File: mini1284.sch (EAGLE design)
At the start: 25 parts, among them U1 ATmega1284P-AU

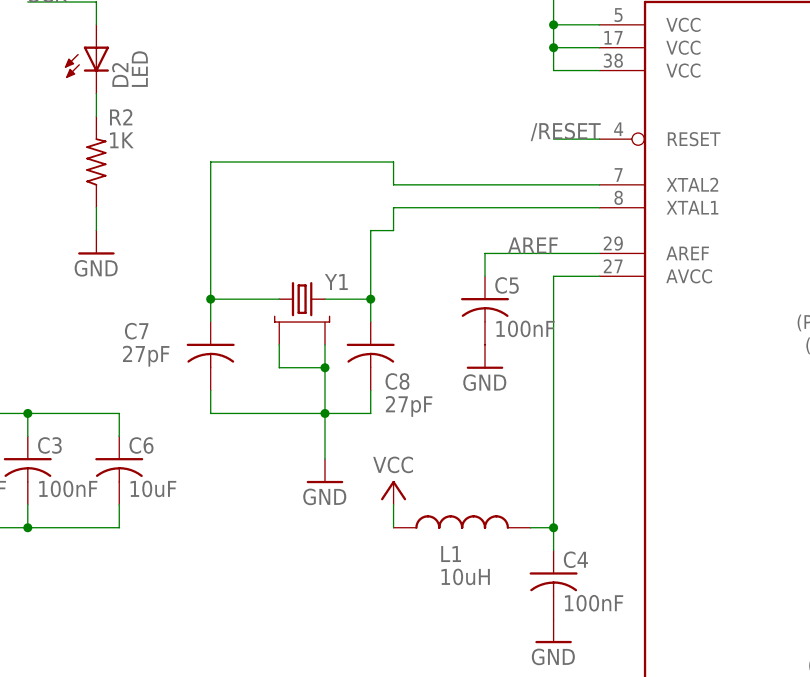
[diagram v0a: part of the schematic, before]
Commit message: Minor tweaks.
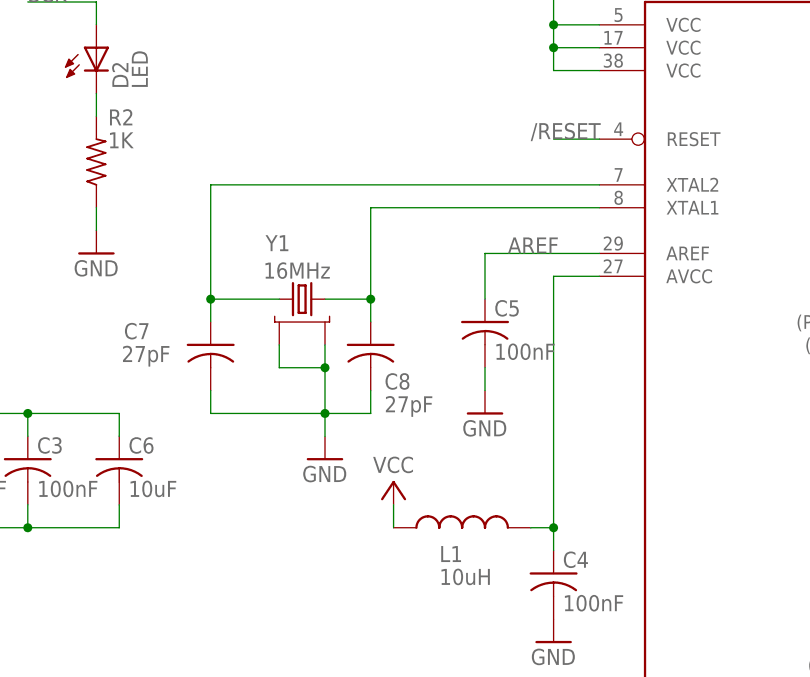
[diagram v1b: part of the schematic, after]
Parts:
- Y1: value (none) -> 16MHz
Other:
- moved on the sheet: C5
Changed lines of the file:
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@@
 <part name="D2" library="_jc" deviceset="LED" device="D0805A" value="LED"/>
 <part name="GND7" library="SparkFun" deviceset="GND" device=""/>
-<part name="Y1" library="_jc" deviceset="CRYSTAL-2GND" device="TSX3225"/>
+<part name="Y1" library="_jc" deviceset="CRYSTAL-2GND" device="TSX3225" value="16MHz"/>
 </parts>
 <sheets>
@@
 <attribute name="VALUE" x="89.916" y="112.649" size="1.778" layer="96"/>
 </instance>
-<instance part="C5" gate="G$1" x="129.54" y="134.62" smashed="yes">
-<attribute name="NAME" x="130.556" y="135.255" size="1.778" layer="95"/>
-<attribute name="VALUE" x="130.556" y="130.429" size="1.778" layer="96"/>
+<instance part="C5" gate="G$1" x="129.54" y="132.08" smashed="yes">
+<attribute name="NAME" x="130.556" y="132.715" size="1.778" layer="95"/>
+<attribute name="VALUE" x="130.556" y="127.889" size="1.778" layer="96"/>
 </instance>
 <instance part="C9" gate="G$1" x="55.88" y="167.64" smashed="yes" rot="R90">
@@
 <attribute name="VALUE" x="117.094" y="115.316" size="1.778" layer="96"/>
 </instance>
-<instance part="GND3" gate="1" x="111.76" y="114.3" smashed="yes">
-<attribute name="VALUE" x="109.22" y="111.76" size="1.778" layer="96"/>
+<instance part="GND3" gate="1" x="111.76" y="116.84" smashed="yes">
+<attribute name="VALUE" x="109.22" y="114.3" size="1.778" layer="96"/>
 </instance>
 <instance part="P+6" gate="VCC" x="68.58" y="129.54" smashed="yes">
@@
 <attribute name="NAME" x="223.52" y="173.99" size="1.778" layer="95" rot="MR0"/>
 </instance>
-<instance part="GND5" gate="1" x="129.54" y="127" smashed="yes">
-<attribute name="VALUE" x="127" y="124.46" size="1.778" layer="96"/>
+<instance part="GND5" gate="1" x="129.54" y="121.92" smashed="yes">
+<attribute name="VALUE" x="127" y="119.38" size="1.778" layer="96"/>
 </instance>
 <instance part="P+7" gate="VCC" x="231.14" y="152.4" smashed="yes">
@@
 <attribute name="VALUE" x="83.82" y="137.16" size="1.778" layer="96"/>
 </instance>
-<instance part="Y1" gate="G$1" x="109.22" y="134.62"/>
+<instance part="Y1" gate="G$1" x="109.22" y="134.62" smashed="yes">
+<attribute name="NAME" x="105.156" y="139.954" size="1.778" layer="95"/>
+<attribute name="VALUE" x="104.902" y="136.906" size="1.778" layer="96"/>
+</instance>
 </instances>
 <busses>
@@
 <wire x1="99.06" y1="124.46" x2="99.06" y2="121.92" width="0.1524" layer="91"/>
 <wire x1="99.06" y1="121.92" x2="111.76" y2="121.92" width="0.1524" layer="91"/>
-<wire x1="111.76" y1="121.92" x2="111.76" y2="116.84" width="0.1524" layer="91"/>
+<wire x1="111.76" y1="121.92" x2="111.76" y2="119.38" width="0.1524" layer="91"/>
 <wire x1="116.84" y1="124.46" x2="116.84" y2="121.92" width="0.1524" layer="91"/>
 <wire x1="116.84" y1="121.92" x2="111.76" y2="121.92" width="0.1524" layer="91"/>
@@
 <pinref part="C5" gate="G$1" pin="2"/>
 <pinref part="GND5" gate="1" pin="GND"/>
+<wire x1="129.54" y1="124.46" x2="129.54" y2="127" width="0.1524" layer="91"/>
 </segment>
 <segment>
@@
 <pinref part="U1" gate="G$1" pin="XTAL1"/>
 <pinref part="C8" gate="G$1" pin="1"/>
-<wire x1="116.84" y1="142.24" x2="119.38" y2="142.24" width="0.1524" layer="91"/>
-<wire x1="119.38" y1="142.24" x2="119.38" y2="144.78" width="0.1524" layer="91"/>
-<wire x1="119.38" y1="144.78" x2="142.24" y2="144.78" width="0.1524" layer="91"/>
+<wire x1="116.84" y1="144.78" x2="142.24" y2="144.78" width="0.1524" layer="91"/>
 <wire x1="116.84" y1="132.08" x2="116.84" y2="134.62" width="0.1524" layer="91"/>
 <pinref part="Y1" gate="G$1" pin="3"/>
-<wire x1="116.84" y1="134.62" x2="116.84" y2="142.24" width="0.1524" layer="91"/>
+<wire x1="116.84" y1="134.62" x2="116.84" y2="144.78" width="0.1524" layer="91"/>
 <wire x1="111.76" y1="134.62" x2="116.84" y2="134.62" width="0.1524" layer="91"/>
 <junction x="116.84" y="134.62"/>
@@
 <segment>
 <pinref part="U1" gate="G$1" pin="XTAL2"/>
-<wire x1="142.24" y1="147.32" x2="119.38" y2="147.32" width="0.1524" layer="91"/>
-<wire x1="119.38" y1="147.32" x2="119.38" y2="149.86" width="0.1524" layer="91"/>
+<wire x1="142.24" y1="147.32" x2="99.06" y2="147.32" width="0.1524" layer="91"/>
 <pinref part="C7" gate="G$1" pin="1"/>
-<wire x1="119.38" y1="149.86" x2="99.06" y2="149.86" width="0.1524" layer="91"/>
-<wire x1="99.06" y1="149.86" x2="99.06" y2="134.62" width="0.1524" layer="91"/>
+<wire x1="99.06" y1="147.32" x2="99.06" y2="134.62" width="0.1524" layer="91"/>
 <wire x1="99.06" y1="134.62" x2="99.06" y2="132.08" width="0.1524" layer="91"/>
 <pinref part="Y1" gate="G$1" pin="1"/>
@@
 <pinref part="C5" gate="G$1" pin="1"/>
 <pinref part="U1" gate="G$1" pin="AREF"/>
-<wire x1="129.54" y1="137.16" x2="129.54" y2="139.7" width="0.1524" layer="91"/>
+<wire x1="129.54" y1="134.62" x2="129.54" y2="139.7" width="0.1524" layer="91"/>
 <wire x1="129.54" y1="139.7" x2="142.24" y2="139.7" width="0.1524" layer="91"/>
 <label x="132.08" y="139.7" size="1.778" layer="95"/>
